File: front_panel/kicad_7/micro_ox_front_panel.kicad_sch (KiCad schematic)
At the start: 8 parts

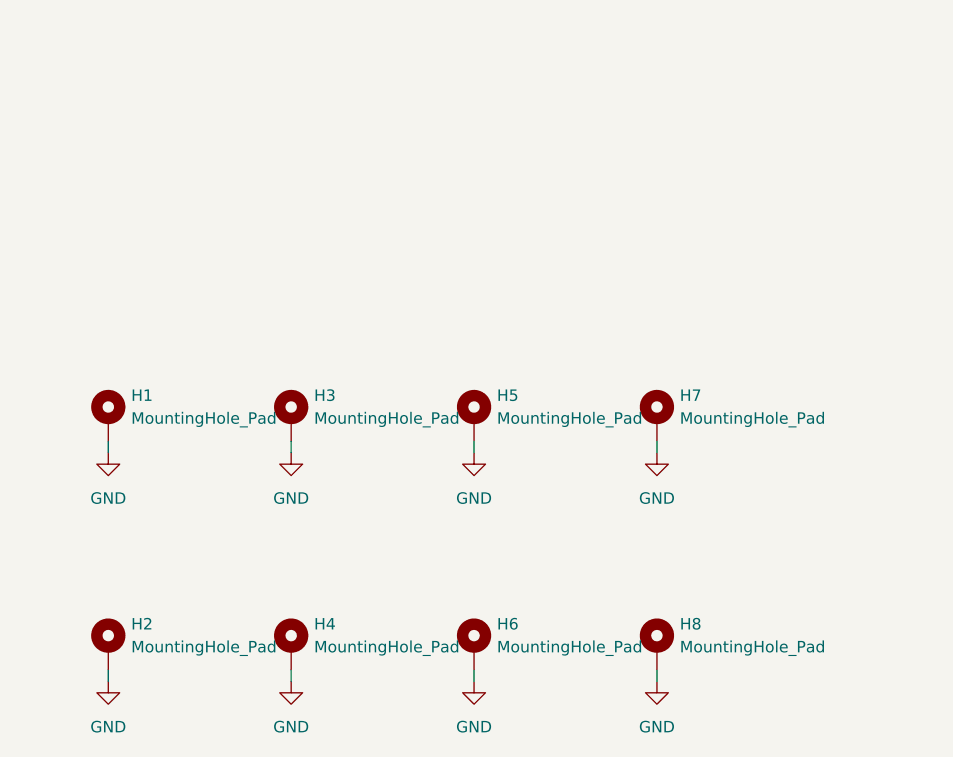
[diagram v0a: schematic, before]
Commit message: Update front panel
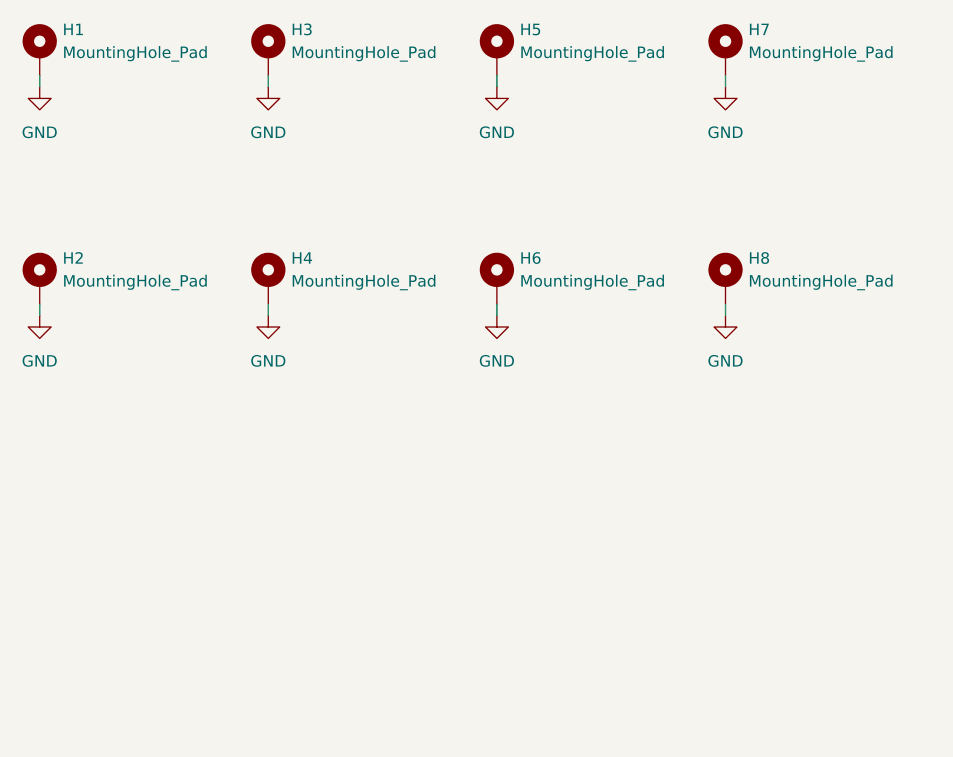
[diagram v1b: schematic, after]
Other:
- moved on the sheet: H1, H2, H3, H4, H5, H6, H7, H8
